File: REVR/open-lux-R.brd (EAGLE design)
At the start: 53 x 68.6 mm, 77 parts, among them IC2 MCP73831, IC3 ATMEGA32U4-AU, IC4 MCP1700-33, Q1 BSS123, Q4 BSS123, T1 FDN340P, T2 FDN340P, X2 USBSMD, X3 8MHz

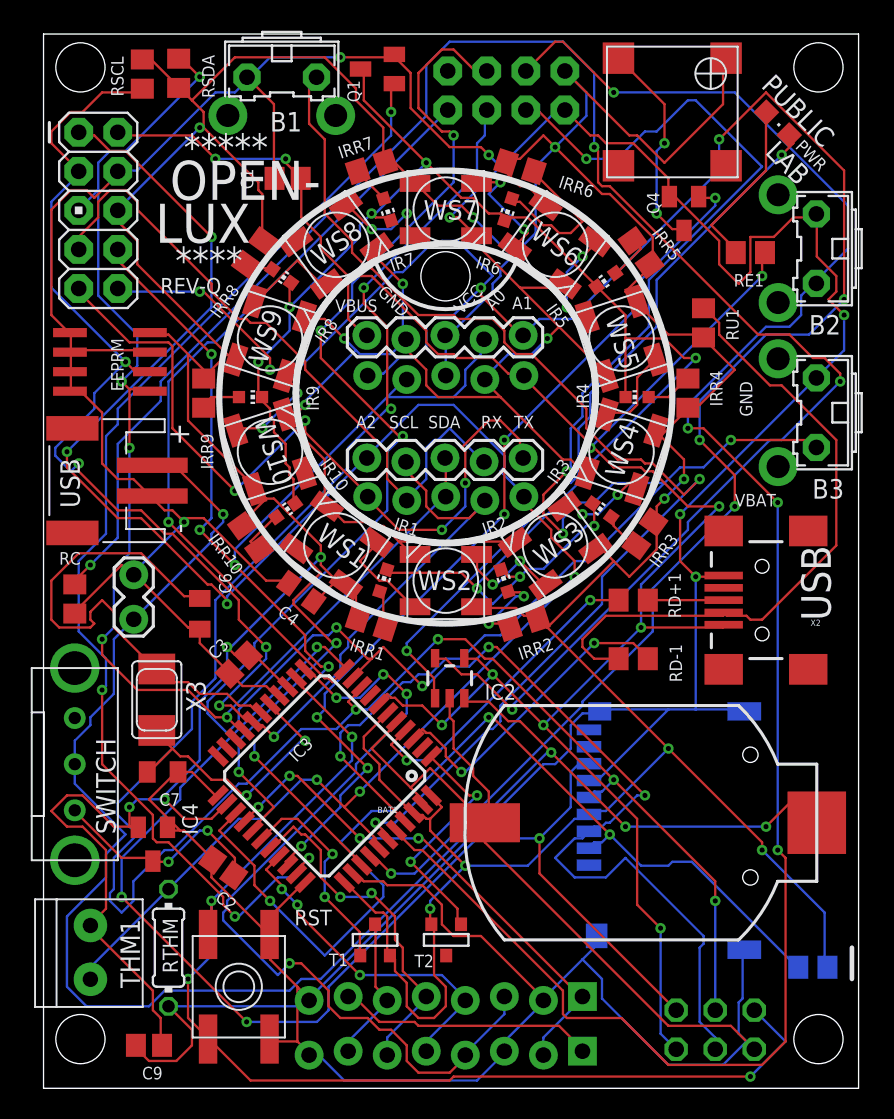
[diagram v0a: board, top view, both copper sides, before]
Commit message: update
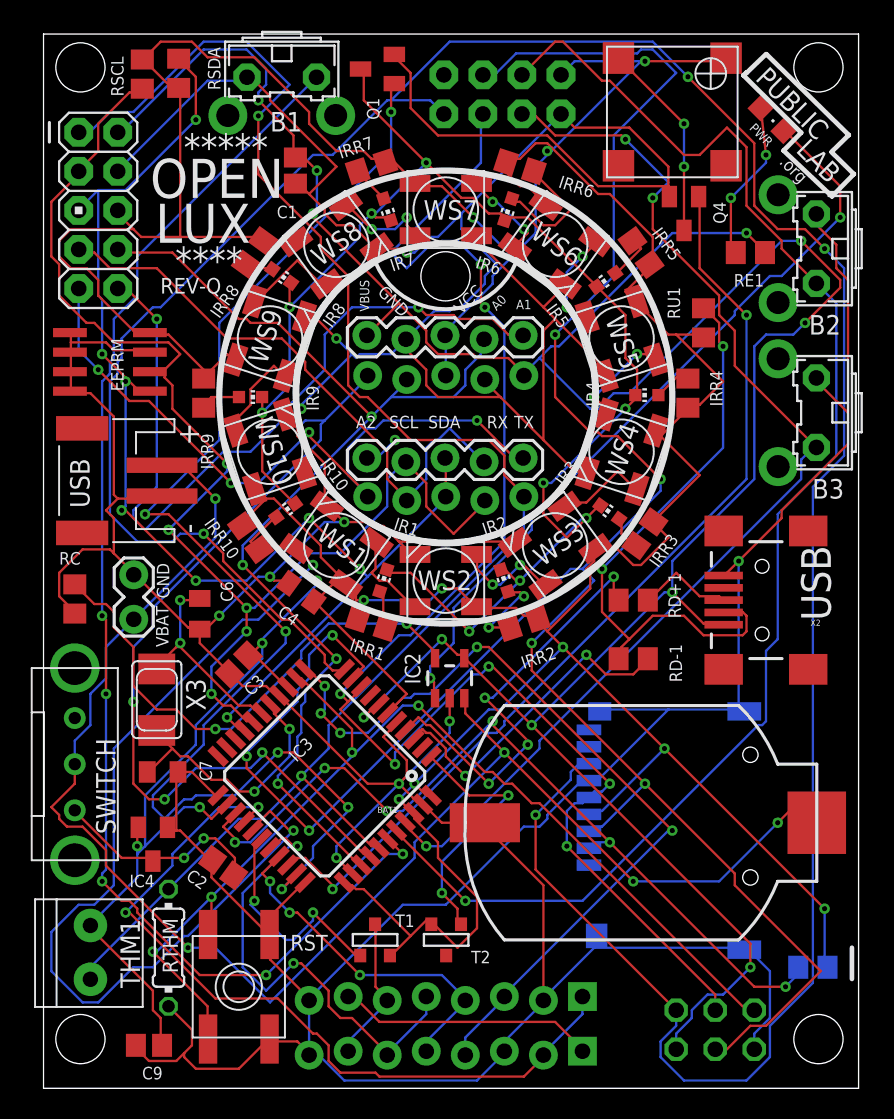
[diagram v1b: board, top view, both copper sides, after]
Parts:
- moved C1 0.72 mm to (16.4, 59.7), turned to 270 degrees
- moved IR4 0.65 mm to (39.2, 45.1)
- moved USB 0.64 mm to (4.01, 39.5)
- moved IR3 0.52 mm to (36.8, 37.5)
- moved PWR 0.46 mm to (47.4, 63.0)
- moved RAD 0.36 mm to (29.8, 64.6)
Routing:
- net N$6: track 121.3 -> 33.7 mm, vias 4 -> 2
- net MISO: track 132.5 -> 186.3 mm, vias 5 -> 4
- net VBUS: track 140.3 -> 181.8 mm, vias 10 -> 11
- net D6: track 25.2 -> 61.1 mm
- net A1: track 142.4 -> 106.7 mm, vias 8 -> 5
- net A5: track 105.5 -> 72.8 mm, vias 5 -> 3
- net SCK: track 131.1 -> 100.8 mm, vias 6 -> 7
- net A4: track 122.3 -> 92.4 mm, vias 4 -> 1
- net GND: track 479.2 -> 454.7 mm, vias 11 -> 10
- net MOSI: track 129.2 -> 150.6 mm
- net N$3: track 33.4 -> 13.8 mm, vias 0 -> 2
- net A2: track 127.7 -> 109.7 mm, vias 6 -> 3
- net D12: track 34.2 -> 50.9 mm, vias 4 -> 2
- net D13: track 75.6 -> 86.9 mm, vias 4 -> 6
- net D4: track 64.5 -> 54.4 mm, vias 3 -> 6
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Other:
- board text added: "(X)"
- board text added: ".org"
- board text added: "A5"
- board text added: "OPEN"
- board text removed: "OPEN-"
